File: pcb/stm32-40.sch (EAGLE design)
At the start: 65 parts, among them IC1 STM32F103RBT6, IC2 CAT24M01WI-GT3, IC3 AMIS30663CANG2G, IC4 MAX487-S, Q1 32768Hz, Q2 8MHz, SW1 KSS-2EG4430, X1 MCV3, X2 MCV3

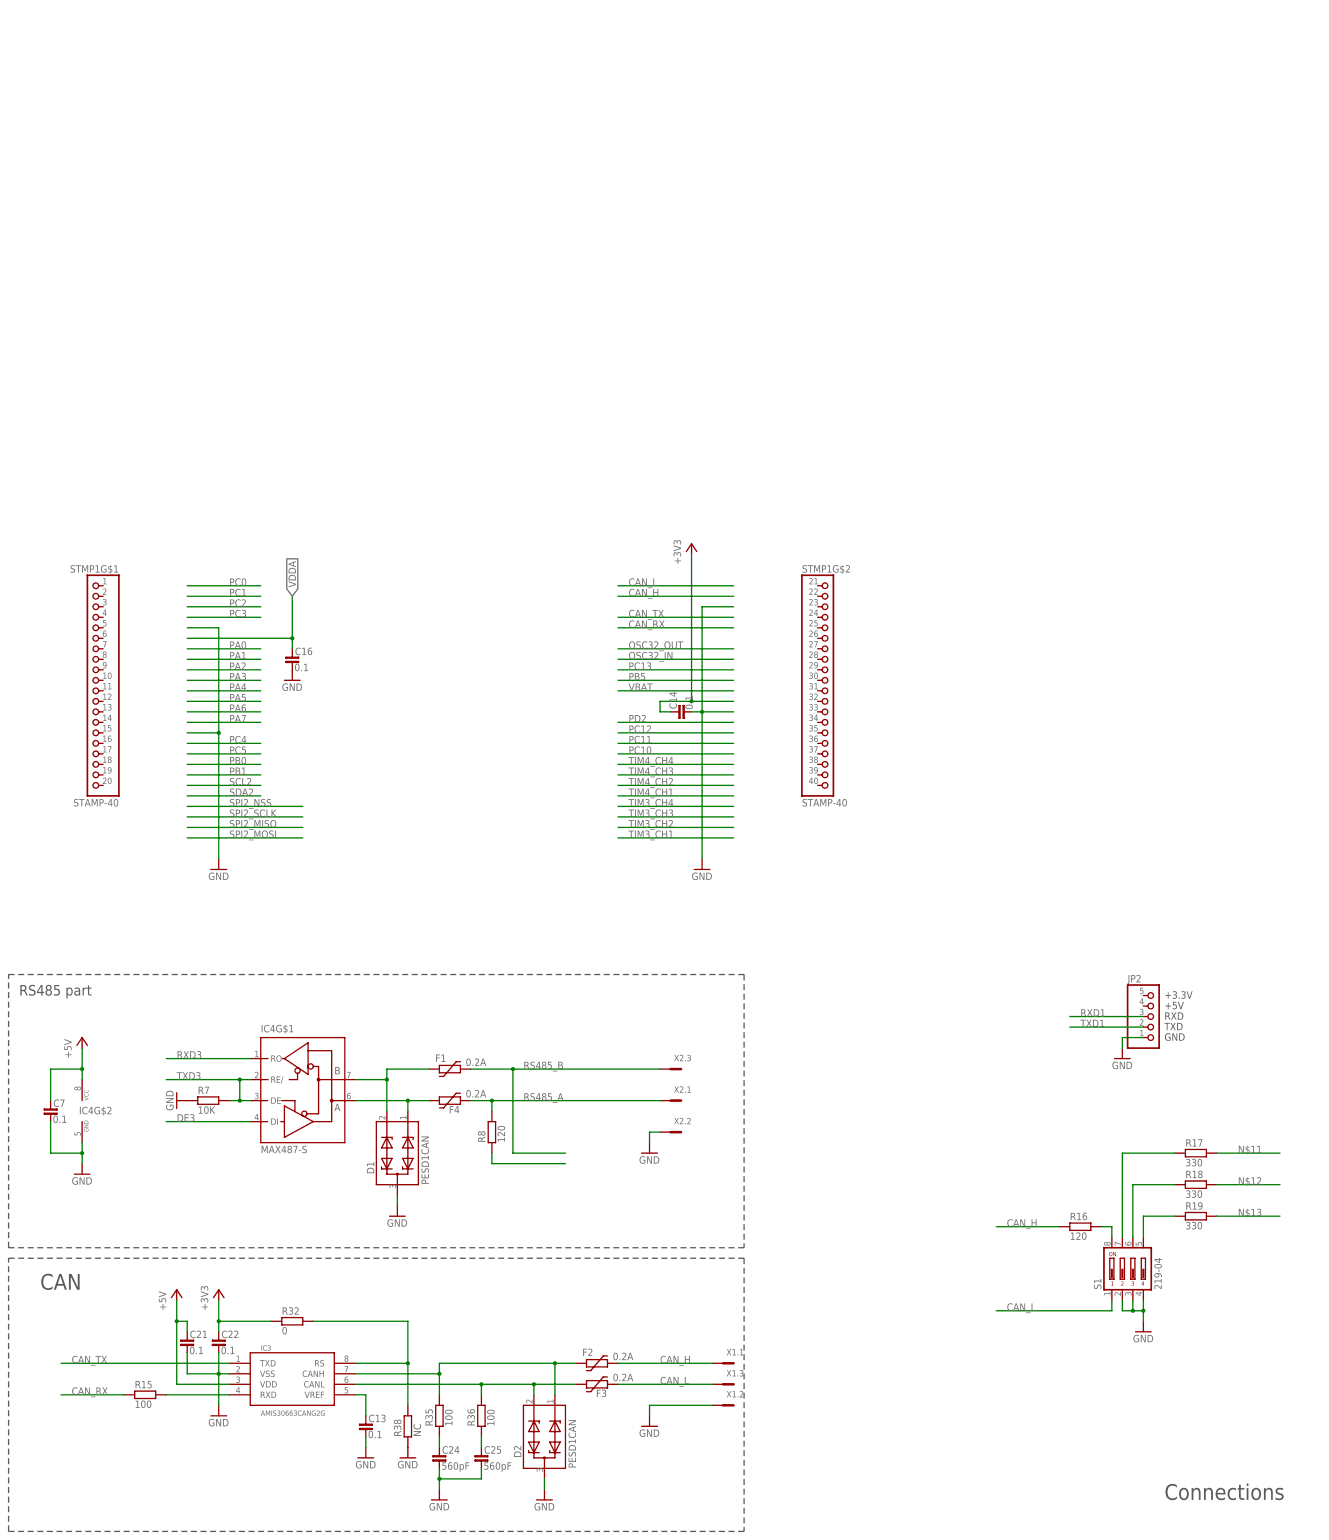
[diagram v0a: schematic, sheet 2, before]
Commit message: route timers
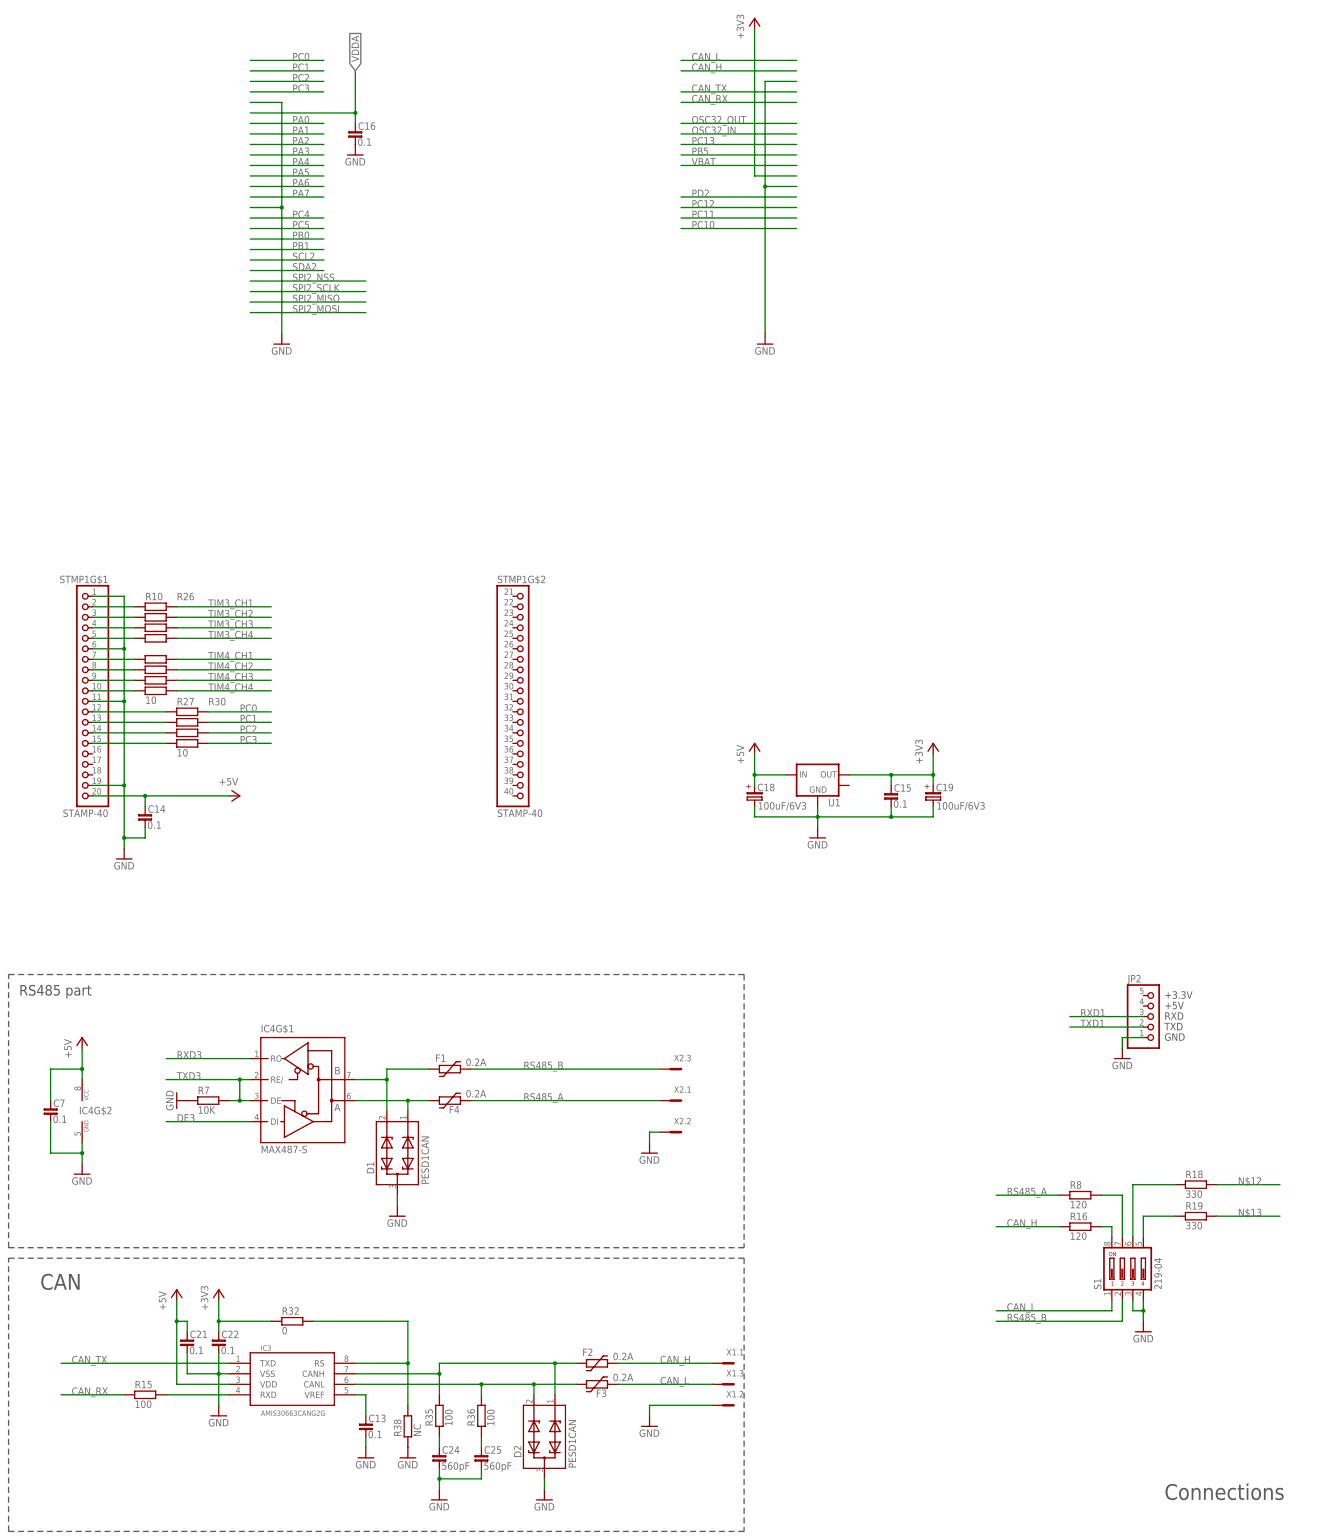
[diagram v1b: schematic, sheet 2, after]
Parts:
- removed R17: 330, rc-master-smd:R_0603
- added C15: 0.1, rc-master-smd:C_0805
- added C18, C19: 100uF/6V3, rc-master-smd:CP_SMCD
- added R10, R11, R12, R22, R23, R24, R25, R26, R27, R28, R29, R30: 10, rc-master-smd:R_0603
- added U1: (no value), vreg-linear:LM1117-3.3
- C14: device rc-master-smd:C_0603 -> rc-master-smd:C_0805
- Q1: device discrete:CRYSTAL-TC26H -> discrete:CRYSTAL-TC38H
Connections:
- removed net N$11: R17.2
- removed net N$14: R8.1
- new net N$15: R10.1, STMP1G$1.2
- new net N$16: R11.1, STMP1G$1.3
- new net N$17: R12.1, STMP1G$1.4
- new net N$18: R22.1, STMP1G$1.5
- new net N$19: R23.1, STMP1G$1.7
- new net N$20: R24.1, STMP1G$1.8
- new net N$21: R25.1, STMP1G$1.9
- new net N$22: R26.1, STMP1G$1.10
- new net N$23: R27.1, STMP1G$1.12
- new net N$24: R28.1, STMP1G$1.13
- new net N$25: R29.1, STMP1G$1.14
- new net N$26: R30.1, STMP1G$1.15
- net +3V3: now also C15.1, C19.+, U1.OUT; no longer C14.1
- net +5V: now also C14.1, C18.+, STMP1G$1.20, U1.IN
- net GND: now also C15.2, C18.-, C19.-, STMP1G$1.1, STMP1G$1.11, STMP1G$1.19, STMP1G$1.6, U1.GND; no longer S1.2
- net N$8: now also R8.2; no longer R17.1
- net PC0: now also R27.2
- net PC1: now also R28.2
- net PC2: now also R29.2
- net PC3: now also R30.2
- net RS485_A: now also R8.1; no longer R8.2
- net RS485_B: now also S1.2
- net TIM3_CH1: now also R10.2
- net TIM3_CH2: now also R11.2
- net TIM3_CH3: now also R12.2
- net TIM3_CH4: now also R22.2
- net TIM4_CH1: now also R23.2
- net TIM4_CH2: now also R24.2
- net TIM4_CH3: now also R25.2
- net TIM4_CH4: now also R26.2
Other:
- moved on the sheet: C14, C16, R8, STMP1G$1, STMP1G$2
